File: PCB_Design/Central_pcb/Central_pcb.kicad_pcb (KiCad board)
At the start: 2 copper layers, 81.8 x 46.5 mm, 54 parts, among them J1 Conn_ARM_JTAG_SWD_10, J2 U.FL-R-SMT_01_, J3 Conn_01x02_Pin, J4 U.FL-R-SMT_01_, J5 SIM, J6 Conn_01x02_Pin, U1 NRF52832-QFAA-R, U2 BQ25171QWDRCRQ1, U3 AMS1117-3.3, U4 BC660K-GL, U5 ESDS304DBVR, Y1 CX2016DB32000D0WZRC1

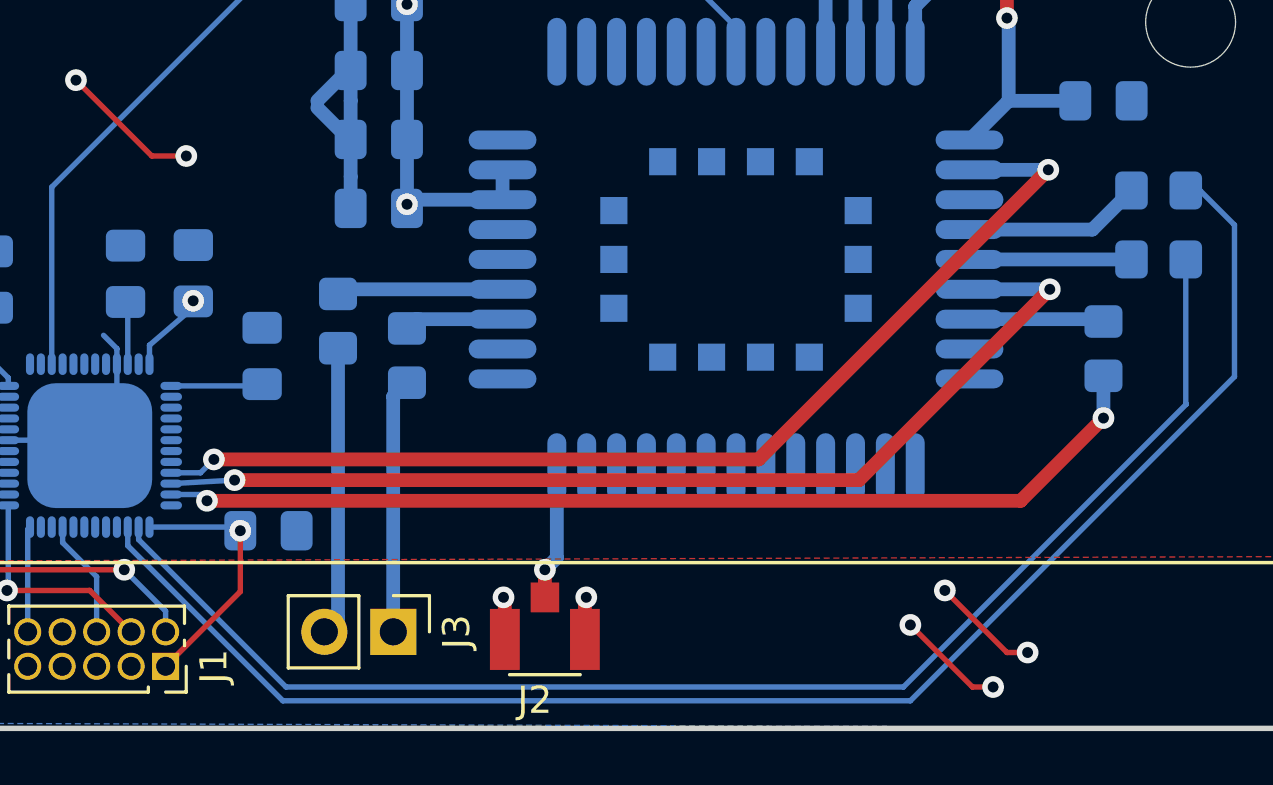
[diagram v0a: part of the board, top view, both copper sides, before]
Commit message: Pcb Update
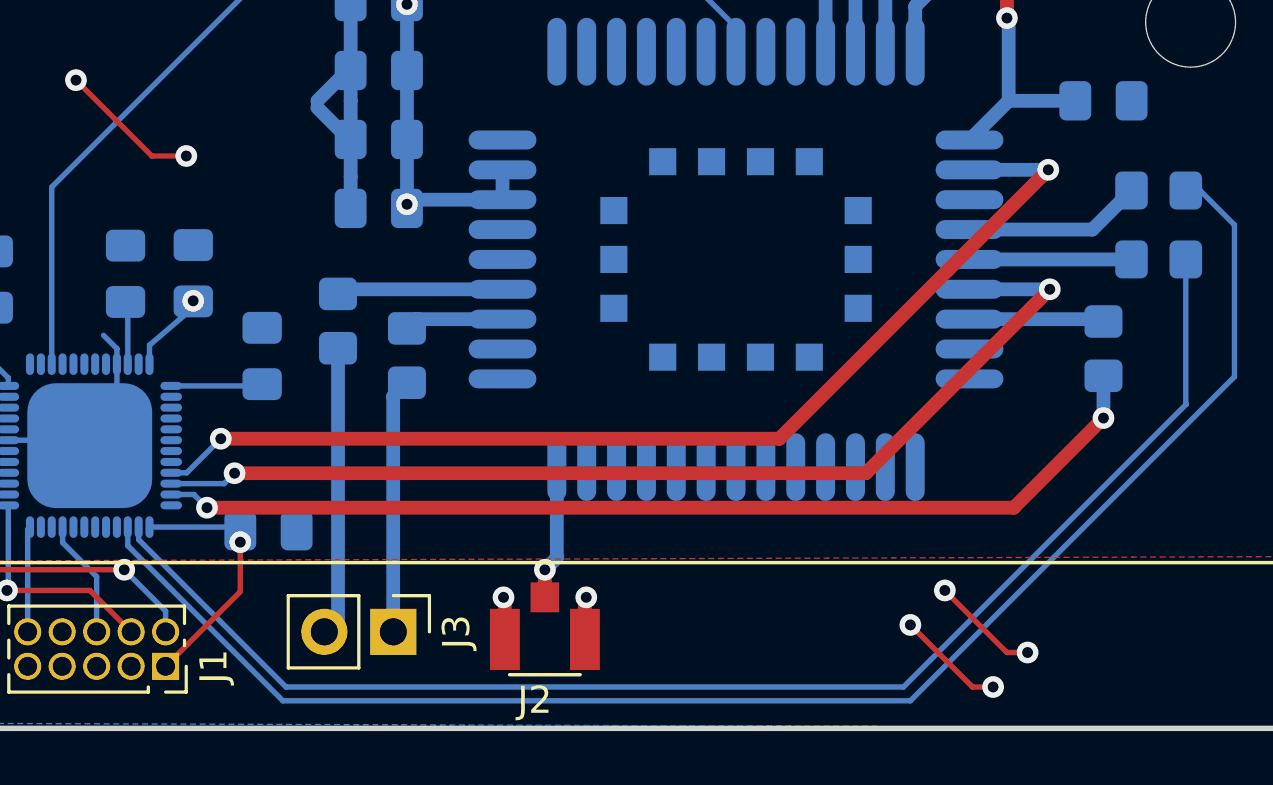
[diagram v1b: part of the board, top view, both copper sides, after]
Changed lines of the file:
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@@
     (pad_to_mask_clearance 0)
     (pcbplotparams
-      (layerselection 0x00010cc_ffffffff)
+      (layerselection 0x00010f0_ffffffff)
       (plot_on_all_layers_selection 0x0000000_00000000)
       (disableapertmacros false)
@@
   )
   (segment (start 175.26 98.378) (end 175.26 79.248) (width 0.508) (layer "B.Cu") (net 1))
-  (segment (start 129.286 112.522) (end 132.036998 109.771002) (width 0.2) (layer "F.Cu") (net 2))
-  (segment (start 132.036998 109.771002) (end 132.036998 107.528) (width 0.2) (layer "F.Cu") (net 2))
+  (segment (start 129.286 112.522) (end 132.037002 109.770998) (width 0.2) (layer "F.Cu") (net 2))
+  (segment (start 132.037002 109.770998) (end 132.037002 107.95) (width 0.2) (layer "F.Cu") (net 2))
   (via (at 130.302 99.06) (size 0.8) (drill 0.4) (layers "F.Cu" "B.Cu") (net 2))
-  (via (at 132.036998 107.528) (size 0.8) (drill 0.4) (layers "F.Cu" "B.Cu") (net 2))
+  (via (at 132.037002 107.95) (size 0.8) (drill 0.4) (layers "F.Cu" "B.Cu") (net 2))
   (via (at 112.776 76.2) (size 0.8) (drill 0.4) (layers "F.Cu" "B.Cu") (net 2))
   (via (at 122.428 100.838) (size 0.8) (drill 0.4) (layers "F.Cu" "B.Cu") (net 2))
@@
   (segment (start 158.896 99.736) (end 163.744 99.736) (width 0.508) (layer "B.Cu") (net 38))
   (segment (start 163.744 99.736) (end 163.83 99.822) (width 0.508) (layer "B.Cu") (net 38))
-  (segment (start 160.782 106.426) (end 130.81 106.426) (width 0.508) (layer "F.Cu") (net 39))
-  (segment (start 163.83 103.378) (end 160.782 106.426) (width 0.508) (layer "F.Cu") (net 39))
-  (via (at 130.81 106.426) (size 0.8) (drill 0.4) (layers "F.Cu" "B.Cu") (net 39))
+  (segment (start 163.83 103.378) (end 160.528 106.68) (width 0.508) (layer "F.Cu") (net 39))
+  (segment (start 160.528 106.68) (end 130.81 106.68) (width 0.508) (layer "F.Cu") (net 39))
+  (via (at 130.81 106.68) (size 0.8) (drill 0.4) (layers "F.Cu" "B.Cu") (net 39))
   (via (at 163.83 103.378) (size 0.8) (drill 0.4) (layers "F.Cu" "B.Cu") (net 39))
   (segment (start 163.83 101.822) (end 163.83 103.378) (width 0.508) (layer "B.Cu") (net 39))
-  (segment (start 130.578 106.194) (end 130.81 106.426) (width 0.2) (layer "B.Cu") (net 39))
-  (segment (start 129.492 106.194) (end 130.578 106.194) (width 0.2) (layer "B.Cu") (net 39))
+  (segment (start 129.492 106.194) (end 130.324 106.194) (width 0.2) (layer "B.Cu") (net 39))
+  (segment (start 130.324 106.194) (end 130.81 106.68) (width 0.2) (layer "B.Cu") (net 39))
   (segment (start 107.688126 82.024228) (end 107.688126 83.065874) (width 0.2) (layer "B.Cu") (net 40))
   (segment (start 104.864 85.89) (end 104.864 89.662) (width 0.2) (layer "B.Cu") (net 40))
@@
   (segment (start 129.492 102.194) (end 132.7775 102.194) (width 0.2) (layer "B.Cu") (net 41))
   (segment (start 132.7775 102.194) (end 132.842 102.1295) (width 0.2) (layer "B.Cu") (net 41))
-  (segment (start 161.798 94.234) (end 151.13 104.902) (width 0.508) (layer "F.Cu") (net 49))
-  (segment (start 151.13 104.902) (end 131.064 104.902) (width 0.508) (layer "F.Cu") (net 49))
-  (via (at 131.064 104.902) (size 0.8) (drill 0.4) (layers "F.Cu" "B.Cu") (net 49))
+  (segment (start 151.892 104.14) (end 131.318 104.14) (width 0.508) (layer "F.Cu") (net 49))
+  (segment (start 161.798 94.234) (end 151.892 104.14) (width 0.508) (layer "F.Cu") (net 49))
+  (via (at 131.318 104.14) (size 0.8) (drill 0.4) (layers "F.Cu" "B.Cu") (net 49))
   (via (at 161.798 94.234) (size 0.8) (drill 0.4) (layers "F.Cu" "B.Cu") (net 49))
   (segment (start 161.796 94.236) (end 161.798 94.234) (width 0.508) (layer "B.Cu") (net 49))
   (segment (start 158.896 94.236) (end 161.796 94.236) (width 0.508) (layer "B.Cu") (net 49))
-  (segment (start 129.492 105.394) (end 130.572 105.394) (width 0.2) (layer "B.Cu") (net 49))
-  (segment (start 130.572 105.394) (end 131.064 104.902) (width 0.2) (layer "B.Cu") (net 49))
+  (segment (start 130.064 105.394) (end 131.318 104.14) (width 0.2) (layer "B.Cu") (net 49))
+  (segment (start 129.492 105.394) (end 130.064 105.394) (width 0.2) (layer "B.Cu") (net 49))
   (segment (start 125.092 101.394) (end 125.092 94.872) (width 0.2) (layer "B.Cu") (net 50))
   (segment (start 134.366 85.598) (end 145.542 85.598) (width 0.2) (layer "B.Cu") (net 50))
@@
   (segment (start 147.32 87.376) (end 148.686 87.376) (width 0.2) (layer "B.Cu") (net 50))
   (segment (start 150.296 88.986) (end 150.296 89.886) (width 0.2) (layer "B.Cu") (net 50))
-  (segment (start 154.824965 105.664) (end 161.852964 98.636001) (width 0.508) (layer "F.Cu") (net 52))
-  (segment (start 131.826 105.664) (end 154.824965 105.664) (width 0.508) (layer "F.Cu") (net 52))
+  (segment (start 161.852964 98.636001) (end 155.078965 105.41) (width 0.508) (layer "F.Cu") (net 52))
+  (segment (start 155.078965 105.41) (end 131.826 105.41) (width 0.508) (layer "F.Cu") (net 52))
   (via (at 161.852964 98.636001) (size 0.8) (drill 0.4) (layers "F.Cu" "B.Cu") (net 52))
-  (via (at 131.826 105.664) (size 0.8) (drill 0.4) (layers "F.Cu" "B.Cu") (net 52))
-  (segment (start 129.492 105.794) (end 131.826 105.664) (width 0.2) (layer "B.Cu") (net 52))
+  (via (at 131.826 105.41) (size 0.8) (drill 0.4) (layers "F.Cu" "B.Cu") (net 52))
+  (segment (start 131.442 105.794) (end 131.826 105.41) (width 0.2) (layer "B.Cu") (net 52))
+  (segment (start 129.492 105.794) (end 131.442 105.794) (width 0.2) (layer "B.Cu") (net 52))
   (segment (start 158.896 98.636) (end 161.852964 98.636001) (width 0.508) (layer "B.Cu") (net 52))
   (segment (start 120.65 107.95) (end 120.142 108.458) (width 0.2) (layer "B.Cu") (net 61))
